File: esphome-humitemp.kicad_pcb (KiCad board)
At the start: 2 copper layers, 47.5 x 31.5 mm, 16 parts, among them J1 eflashy32, J2 USB_IN, J3 USB_OUT, U1 SHT35-DISB, U2 TLV75533PDBV, U3 ESP32-WROOM-32D

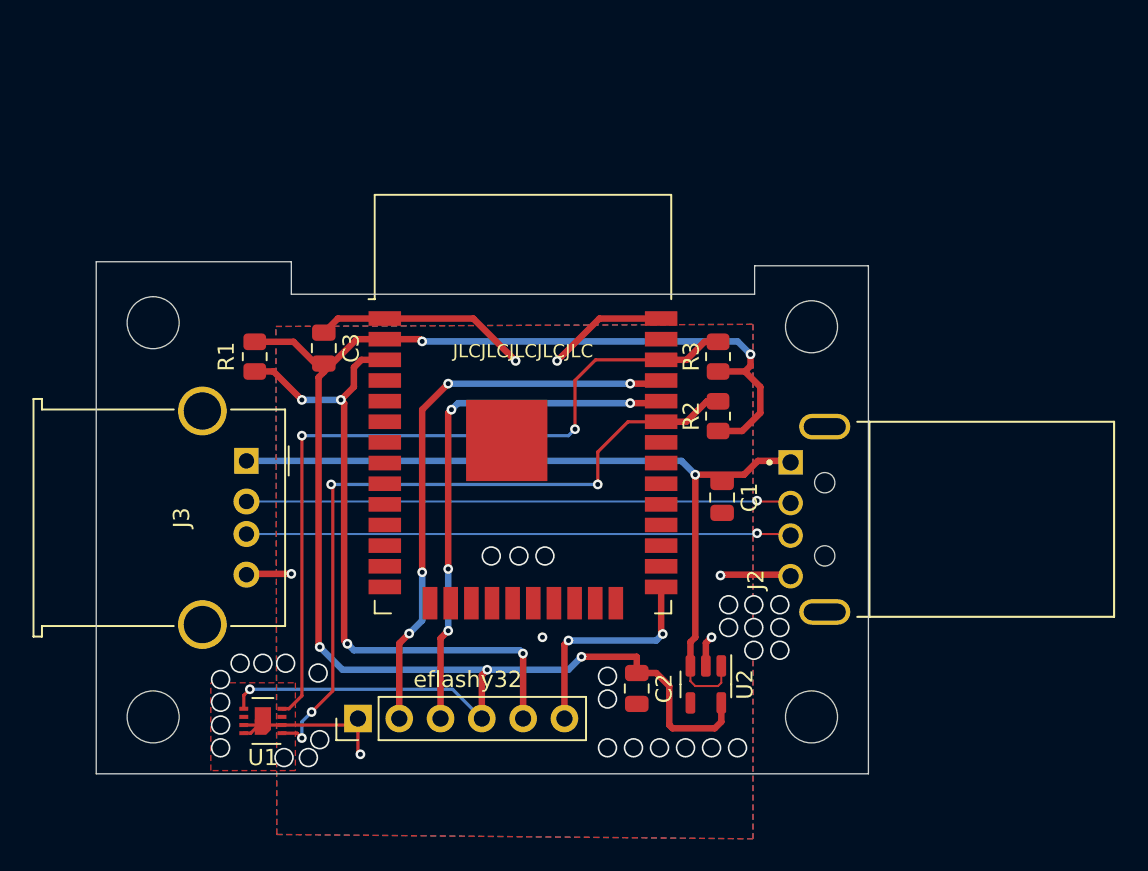
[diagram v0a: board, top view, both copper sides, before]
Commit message: v2 ecad
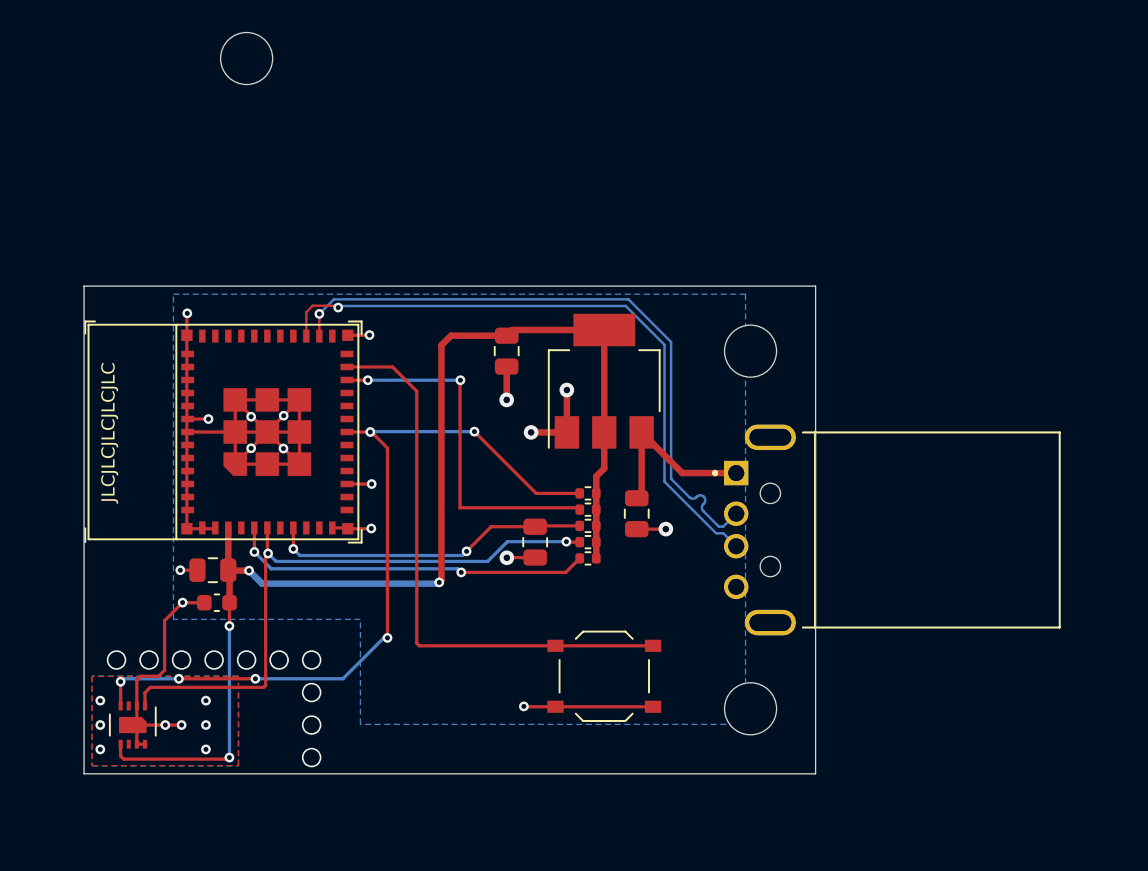
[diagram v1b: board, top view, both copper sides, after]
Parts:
- removed C3: 10uF, Capacitor_SMD:C_0805_2012Metric
- removed H3: MountingHole, MountingHole:MountingHole_3.2mm_M3
- removed J1: eflashy32, Connector_PinHeader_2.54mm:PinHeader_1x06_P2.54mm_Vertical
- removed J3: USB_OUT, Connector_USB:USB_A_Molex_67643_Horizontal
- removed R1: 10k, Resistor_SMD:R_0805_2012Metric
- removed U2: TLV75533PDBV, Package_TO_SOT_SMD:SOT-23-5
- added C4: 10u, Capacitor_SMD:C_0805_2012Metric, F.Cu at (117.8, 65.8)
- added C5: 0.1u, Capacitor_SMD:C_0603_1608Metric, F.Cu at (98.2, 69.5)
- added C6: 10u, Capacitor_SMD:C_0805_2012Metric, F.Cu at (97.9, 67.5)
- added R4: 10k, Resistor_SMD:R_0402_1005Metric, F.Cu at (121.0, 64.8)
- added R5: 10k, Resistor_SMD:R_0402_1005Metric, F.Cu at (121.0, 66.8)
- added R6: 10k, Resistor_SMD:R_0402_1005Metric, F.Cu at (121.0, 63.8)
- added SW1: RESET, Button_Switch_SMD:SW_Push_1P1T_XKB_TS-1187A, F.Cu at (122.0, 74.0)
- added U4: ESP32-C3-MINI-1, Espressif:ESP32-C3-MINI-1, F.Cu at (98.6, 59.0)
- R2, R3: footprint Resistor_SMD:R_0805_2012Metric -> Resistor_SMD:R_0402_1005Metric
- U1: value SHT35-DISB -> SHT3x
- U3: value ESP32-WROOM-32D -> AMS1117-3.3; footprint RF_Module:ESP32-WROOM-32 -> Package_TO_SOT_SMD:SOT-223-3_TabPin2
- moved C2 22.2 mm to (116.0, 54.0)
- moved H4 17.2 mm to (100.0, 36.0)
- moved R3 11.6 mm to (121.0, 62.8), turned to 180 degrees
- moved R2 11.1 mm to (121.0, 65.8), turned to 180 degrees
- moved U1 8.00 mm to (93.0, 77.0), turned to -90 degrees
- moved U3 6.66 mm to (122.0, 55.9), turned to 90 degrees
- moved C1 5.34 mm to (124.0, 64.0)
- moved H1 4.04 mm to (131.0, 54.0)
- moved H2 3.78 mm to (131.0, 76.0)
- moved J2 3.41 mm to (132.2, 65.0)
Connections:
- J2 pad 2: Net-(J2-Pad2) -> D-
- J2 pad 3: Net-(J2-Pad3) -> D+
- U1 pad 3: (no net) -> unconnected-(U1-ALERT-Pad3)
- U1 pad 6: (no net) -> unconnected-(U1-~{RESET}-Pad6)
- U3 pad 3: /EN -> VBUS
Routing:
- net GND: track 40.8 -> 90.4 mm, vias 37 -> 25
- net VBUS: track 50.3 -> 11.0 mm, vias 1 -> 0
- net D+: track 0.00 -> 39.2 mm, vias 0 -> 1
- net D-: track 0.00 -> 39.2 mm, vias 0 -> 1
- net /TXD: track 35.0 -> 0.00 mm, vias 4 -> 0
- net +3V3: track 108.7 -> 74.4 mm, vias 6 -> 4
- net Net-(J2-Pad3): track 33.4 -> 0.00 mm, vias 1 -> 0
- net Net-(J2-Pad2): track 33.4 -> 0.00 mm, vias 1 -> 0
- net /RXD: track 32.4 -> 0.00 mm, vias 4 -> 0
- net Net-(U4-GPIO2/ADC1_CH2): track 0.00 -> 22.4 mm, vias 0 -> 2
- net Net-(U4-GPIO8): track 0.00 -> 22.3 mm, vias 0 -> 2
- net /GPIO0: track 13.8 -> 35.0 mm, vias 2 -> 0
- net /EN: track 40.7 -> 19.8 mm, vias 4 -> 2
- net SDA: track 44.9 -> 38.1 mm, vias 4 -> 2
- net SCL: track 47.3 -> 48.1 mm, vias 2 -> 6
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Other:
- board size 47.5 x 31.5 mm -> 45 x 30 mm
- board text added: "<<hash>>"
- board text added: "esphome-humitemp v2"
- board text removed: "esphome-humitemp v1"
